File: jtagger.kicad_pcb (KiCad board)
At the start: 4 copper layers, 63 x 32 mm, 106 parts, among them J1 µUSB, J2 ARM_JTAG, J3 PADS, Q1 IRLML6402, Q2 IRLML6402, Q3 MMBT3906, Q4 2N7002, U1 MCP1700T-3302E/TT, U10 TPS61045DRB, U11 SI8642-QSOP, U2 SI8645-QSOP, U3 FT2232HQ, U4 EPM240-TQFP100, U5 MCP1700T-3302E/TT, U6 REE-0505S, U7 OSC-50MHz, U8 LTC1844ES5-3.3, U9 DG449DS, X1 12 MHz

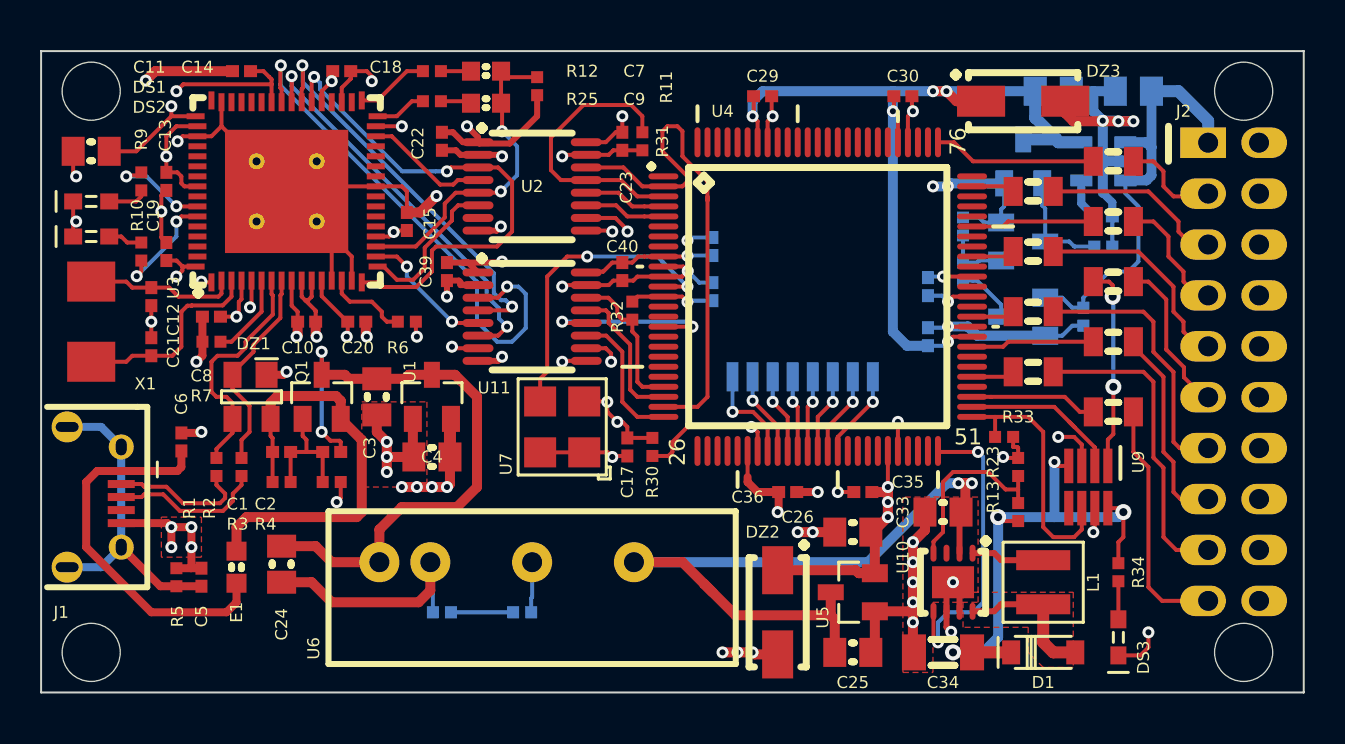
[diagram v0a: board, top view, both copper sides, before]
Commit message: Version submitted to fab
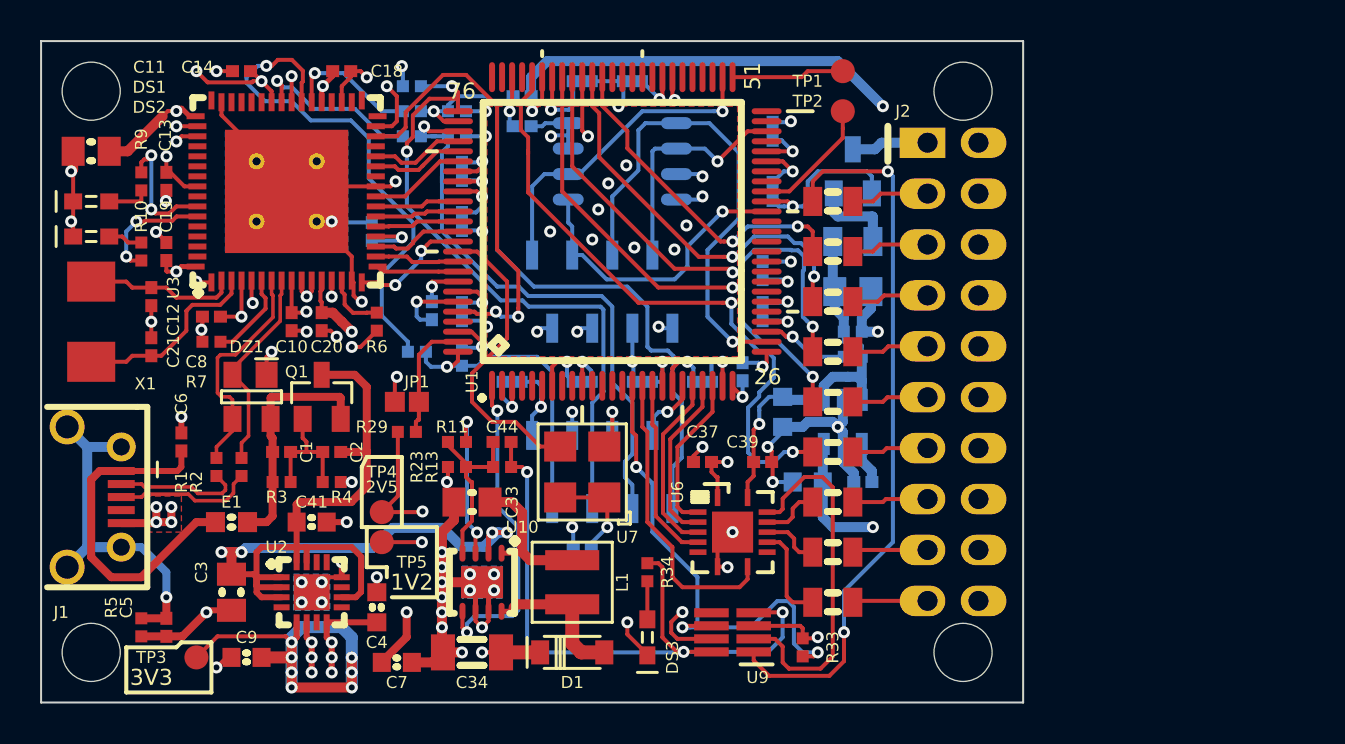
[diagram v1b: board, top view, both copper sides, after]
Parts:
- removed DZ2, DZ3: 1SMA5914BT3G, IPC7351-Nominal:DIOM5226X203
- removed Q3: MMBT3906, smd-semi:SOT-23
- removed Q4: 2N7002, smd-semi:SOT-23
- removed R32: 3k3, IPC7351-Nominal:RESC1005X40
- removed U11: SI8642-QSOP, IPC7351-Nominal:SOP63P600X160-16
- removed U8: LTC1844ES5-3.3, smd-semi:SOT-23-5
- added C41: 1u, IPC7351-Nominal:CAPC1608X55, F.Cu at (113.5, 111.5)
- added C42: 100n, IPC7351-Nominal:CAPC1005X55, B.Cu at (136.5, 95.0)
- added C43: 100n, IPC7351-Nominal:CAPC1005X55, B.Cu at (127.0, 89.5)
- added C44: 47p, IPC7351-Nominal:CAPC1005X55, F.Cu at (123.0, 107.5)
- added C45: 1u, IPC7351-Nominal:CAPC1608X55, B.Cu at (137.0, 106.0)
- added C46: 100n, IPC7351-Nominal:CAPC1005X55, B.Cu at (141.0, 109.5)
- added C47: 100n, IPC7351-Nominal:CAPC1005X55, B.Cu at (127.0, 112.8)
- added G***: LOGO, LOGO, B.Cu at (106.5, 109.0)
- added J4: JTAG, conn-molex:CONN-MOLEX-52808-0871, B.Cu at (128.0, 109.0)
- added JP1: PROGB, JUMPER-SOLDER, F.Cu at (118.2, 105.5)
- added R35: 10k, IPC7351-Nominal:RESC1005X40, B.Cu at (140.5, 102.0)
- added TP1: DONE, conn-test:TEST-SMD-SMALL, F.Cu at (140.0, 89.0)
- added TP2: INITB, conn-test:TEST-SMD-SMALL, F.Cu at (140.0, 91.0)
- added TP3: DONE, conn-test:TEST-SMD-SMALL, F.Cu at (107.8, 118.2)
- added TP4: DONE, conn-test:TEST-SMD-SMALL, F.Cu at (117.0, 111.0)
- added TP5: DONE, conn-test:TEST-SMD-SMALL, F.Cu at (117.0, 112.5)
- C12, C21: value 15p -> 3p3
- C15, C17, C22, C23, C29, C30, C35, C36, C40, R30: moved to B.Cu
- C24: value 10u -> 1u; footprint IPC7351-Nominal:CAPC2012X70 -> IPC7351-Nominal:CAPC1608X55; moved to B.Cu
- C25, C26: value 10u -> 100n; footprint IPC7351-Nominal:CAPC2012X70 -> IPC7351-Nominal:CAPC1005X55; moved to B.Cu
- C27: value 10u -> 100n; footprint IPC7351-Nominal:CAPC2012X70 -> IPC7351-Nominal:CAPC1005X55
- C37: moved to F.Cu
- C4: value 10u -> 1u; footprint IPC7351-Nominal:CAPC2012X70 -> IPC7351-Nominal:CAPC1608X55
- C7: value 100p -> 1u
- C9: value 1n -> 1u
- DS3: value LED-0603 -> LED
- DZ1: value SP0503BAHT -> DRTR5V0U2SR
- J3: value PADS -> FLASH
- R12: value 1k -> 10k; moved to B.Cu
- R13: value R-0402 -> 1M
- R23: value R-0402 -> 200k
- R24, R8: value 1M -> 0R
- R25: value 1k -> THERM; footprint IPC7351-Nominal:RESC1005X40 -> IPC7351-Nominal:RESC2012X50; moved to B.Cu
- R26, R27: value 3k3 -> 0R
- R28: value 3k3 -> 1k
- R29: value 3k3 -> 1k; moved to F.Cu
- R31: value 3k3 -> 1k; moved to B.Cu
- U1: value MCP1700T-3302E/TT -> XC3S50-VQ100; footprint smd-semi:SOT-23 -> IPC7351-Nominal:QFP50P1600X1600X100-100
- U2: value SI8645-QSOP -> ADP322ACPZ-145; footprint IPC7351-Nominal:SOP63P600X160-16 -> IPC7351-Nominal:QFN50P300X300X100-17
- U4: value EPM240-TQFP100 -> S25FL204; footprint IPC7351-Nominal:QFP50P1600X1600X160-100 -> IPC7351-Nominal:SOIC127P600X175-8; moved to B.Cu
- U5: value MCP1700T-3302E/TT -> LTC1844ES5-3.3; footprint smd-semi:SOT-23 -> smd-semi:SOT-23-5; moved to B.Cu
- U6: value REE-0505S -> TXB0104RGY; footprint manuf:RECOM-REE-0505S -> manuf:TEXAS-RGY
- moved R29 34.2 mm to (118.2, 107.0), turned to 0 degrees
- moved R28 32.9 mm to (120.8, 91.0)
- moved C27 32.9 mm to (119.5, 101.0), turned to 270 degrees
- moved C9 30.1 mm to (110.2, 118.2)
- moved C7 29.8 mm to (117.8, 118.5), turned to 0 degrees
- moved R26 28.4 mm to (118.5, 89.8), turned to 180 degrees
- moved R27 28.3 mm to (118.5, 92.2), turned to 180 degrees
- moved R23 28.0 mm to (120.8, 108.8), turned to 180 degrees
- moved C24 26.6 mm to (138.2, 109.5), turned to 180 degrees
- moved R13 25.8 mm to (123.0, 108.8), turned to 180 degrees
- moved R12 25.4 mm to (140.5, 103.2), turned to 0 degrees
- moved C26 25.0 mm to (129.5, 89.5)
- moved R8 25.0 mm to (118.5, 91.0), turned to 180 degrees
- moved C28 24.4 mm to (130.0, 104.5), turned to 180 degrees
- moved C31 24.0 mm to (121.0, 94.0)
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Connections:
- net /IN_OE renamed /AD11
- net Net-(U3-Pad26) renamed /AD8
- net Net-(U3-Pad34) renamed /AD15
- C16 pad 1: /VT_IN -> +VTGT
- C16 pad 2: (GND) -> GND
- C17 pad 1: (+3.3) -> /VTGTLIM
- C17 pad 2: (GND) -> GND
- C23 pad 1: (+3.3) -> +3.3
- C23 pad 2: (GND) -> GND
- C24 pad 1: +5 -> /VTGTLIM
- C25 pad 1: (+5) -> +2.5
- C25 pad 2: (GND) -> GND
- C26 pad 1: (+3.3) -> +2.5
- C26 pad 2: (GND) -> GND
- C27 pad 1: (+VTGT) -> +1.2
- C27 pad 2: (GND) -> GND
- C28 pad 1: Net-(C28-Pad1) -> +1.2
- C28 pad 2: (GND) -> GND
- C29 pad 1: (+VTGT) -> +3.3
- C29 pad 2: (GND) -> GND
- C30 pad 1: (+VTGT) -> +2.5
- C30 pad 2: (GND) -> GND
- C31 pad 1: (+3.3) -> +3.3
- C31 pad 2: (GND) -> GND
- C32 pad 1: (+VTGT) -> +2.5
- C32 pad 2: (GND) -> GND
- C33 pad 1: (+5) -> /SWL
- C33 pad 2: (GND) -> GND
- C34 pad 2: (GND) -> GND
- C35 pad 1: (+3.3) -> +3.3
- C35 pad 2: (GND) -> GND
- C36 pad 1: (+3.3) -> +3.3
- C36 pad 2: (GND) -> GND
- C37 pad 1: (+3.3) -> +3.3
- C37 pad 2: (GND) -> GND
- C38 pad 1: (+3.3) -> +3.3
- C38 pad 2: (GND) -> GND
- C39 pad 1: +3.3 -> +VTGT
- C4 pad 1: +3.3 -> +1.2
- C40 pad 1: (+3.3) -> +3.3
- C40 pad 2: (GND) -> GND
- C7 pad 1: /IN_TMS -> +2.5
- C7 pad 2: Net-(C7-Pad2) -> GND
- C9 pad 1: /IN_TMS -> +3.3
- C9 pad 2: Net-(C9-Pad2) -> GND
- DS3 pad 1: (GND) -> GND
- J2 pad 1: /VT_IN -> Net-(J2-Pad1)
- J2 pad 10: (GND) -> GND
- J2 pad 12: (GND) -> GND
- J2 pad 14: (GND) -> GND
- J2 pad 16: (GND) -> GND
- J2 pad 18: (GND) -> GND
- J2 pad 20: (GND) -> GND
- J2 pad 4: (GND) -> GND
- J2 pad 6: (GND) -> GND
- J2 pad 8: (GND) -> GND
- J3 pad 1: Net-(J3-Pad1) -> /CCLK
- J3 pad 2: Net-(J3-Pad2) -> +3.3
- J3 pad 3: Net-(J3-Pad3) -> /SPIMOSI
- J3 pad 4: Net-(J3-Pad4) -> GND
- J3 pad 5: Net-(J3-Pad5) -> /SPI#CS
- J3 pad 6: Net-(J3-Pad6) -> GND
- J3 pad 7: Net-(J3-Pad7) -> /SPIMISO
- J3 pad 8: Net-(J3-Pad8) -> GND
- Q2 pad 1: Net-(Q2-Pad1) -> GND
- Q2 pad 2: (+3.3) -> Net-(Q2-Pad2)
- Q2 pad 3: (+VTGT) -> Net-(J2-Pad1)
- R11 pad 1: +3.3 -> Net-(C44-Pad2)
- R11 pad 2: /IN_TMS -> Net-(R11-Pad2)
- R12 pad 1: Net-(C7-Pad2) -> /TGTSENSE
- R12 pad 2: Net-(R12-Pad2) -> +VTGT
- R13 pad 2: Net-(R13-Pad2) -> Net-(C44-Pad2)
- R14 pad 2: /TARG_#TRST -> Net-(R14-Pad2)
- R15 pad 2: /TARG_TDI -> /IN_TDI
- R16 pad 2: /TARG_TMS -> /IN_TMS
- R17 pad 2: /TARG_TCLKO -> /IN_TCK
- R18 pad 2: /AUX1_HVP -> /IN_RTCK
- R19 pad 2: /TARG_TDO -> /IN_TDO
- R20 pad 2: /TARG_#SRST -> Net-(R20-Pad2)
- R21 pad 2: /TARG_DBGREQ -> Net-(R21-Pad2)
- R22 pad 2: /TARG_DBGACK -> Net-(R22-Pad2)
- R23 pad 1: Net-(R13-Pad2) -> Net-(C44-Pad2)
- R23 pad 2: (GND) -> GND
- R24 pad 1: Net-(R24-Pad1) -> /FPGA_TDI
- R24 pad 2: (GND) -> Net-(R24-Pad2)
- R25 pad 1: Net-(C9-Pad2) -> Net-(Q2-Pad2)
- R25 pad 2: Net-(R25-Pad2) -> +VTGT
- R26 pad 1: (+3.3) -> /FPGA_TDO
- R26 pad 2: Net-(Q3-Pad1) -> Net-(R26-Pad2)
- R27 pad 1: Net-(Q3-Pad1) -> /FPGA_TMS
- R27 pad 2: Net-(Q4-Pad3) -> Net-(R27-Pad2)
- R28 pad 1: Net-(Q2-Pad1) -> /FPGA_TCK
- R28 pad 2: (GND) -> GND
- R29 pad 1: /VT_IN -> +2.5
- R29 pad 2: (GND) -> Net-(JP1-Pad1)
- R30 pad 1: /PC_TCK -> +3.3
- R30 pad 2: (GND) -> /FPGA_TMS
- R31 pad 1: /CPLD_SEL -> +3.3
- R31 pad 2: (GND) -> /FPGA_TDI
- R33 pad 1: Net-(R33-Pad1) -> /VPPEN
- R33 pad 2: (GND) -> GND
- R8 pad 1: GND -> /FPGA_TCK
- R8 pad 2: Net-(R24-Pad1) -> Net-(R8-Pad2)
- U1 pad 1: GND -> /VCTRL
- U1 pad 2: +3.3 -> Net-(U1-Pad2)
- U1 pad 3: +5 -> GND
- U10 pad 2: (+5) -> +5
- U10 pad 3: Net-(U10-Pad3) -> Net-(R11-Pad2)
- U10 pad 4: Net-(R13-Pad2) -> Net-(C44-Pad2)
- U10 pad 6: (GND) -> GND
- U10 pad 7: (GND) -> GND
- U10 pad 9: (GND) -> GND
- U2 pad 1: +3.3 -> +5
- U2 pad 10: (+3.3) -> +5
- U2 pad 11: /PC_TDI -> (no net)
- U2 pad 12: /PC_TMS -> GND
- U2 pad 13: /CPLD_SEL -> (no net)
- U2 pad 14: /PC_TCK -> (no net)
- U2 pad 15: (GND) -> +5
- U2 pad 16: (+3.3) -> +5
- U2 pad 2: GND -> +5
- U2 pad 3: /IN_TCK -> +5
- U2 pad 4: /IN_CPLD_SEL -> (no net)
- U2 pad 5: /IN_TMS -> +3.3
- U2 pad 6: /IN_TDI -> +2.5
- U2 pad 8: GND -> +1.2
- U2 pad 9: (GND) -> (no net)
- U3 pad 16: /IN_TCK -> /AD0
- U3 pad 17: /IN_TDI -> /AD1
- U3 pad 18: /IN_TDO -> /AD2
- U3 pad 19: /IN_TMS -> /AD3
- U3 pad 21: Net-(U3-Pad21) -> /AD4
- U3 pad 22: Net-(U3-Pad22) -> /AD5
- U3 pad 23: Net-(U3-Pad23) -> /AD6
- U3 pad 24: Net-(U3-Pad24) -> /AD7
- U3 pad 27: Net-(U3-Pad27) -> /AD9
- U3 pad 28: Net-(U3-Pad28) -> /AD10
- U3 pad 30: /IN_CPLD_SEL -> /AD12
- U3 pad 32: Net-(R25-Pad2) -> /AD13
- U3 pad 33: Net-(R12-Pad2) -> /AD14
- U3 pad 38: /IN_TCK -> Net-(R8-Pad2)
- U3 pad 39: /IN_CPLD_TDI -> Net-(R24-Pad2)
- U3 pad 40: /IN_CPLD_TDO -> Net-(R26-Pad2)
- U3 pad 41: /IN_CPLD_TMS -> Net-(R27-Pad2)
- U4 pad 1: Net-(U4-Pad1) -> /SPI#CS
- U4 pad 2: /PC_TCK -> /SPIMISO
- U4 pad 3: /CPLD_SEL -> +3.3
- U4 pad 4: /PC_TMS -> GND
- U4 pad 5: /PC_TDI -> /SPIMOSI
- U4 pad 6: Net-(U4-Pad6) -> /CCLK
- U4 pad 7: Net-(U4-Pad7) -> +3.3
- U4 pad 8: Net-(U4-Pad8) -> +3.3
- U5 pad 1: (GND) -> +VTGT
- U5 pad 2: (+3.3) -> GND
- U5 pad 3: (+5) -> +VTGT
- U6 pad 1: +5 -> +3.3
- U6 pad 2: GND -> /IN_#TRST
- U6 pad 4: (GND) -> /IN_DBGREQ
- U6 pad 6: (+5) -> (no net)
- U7 pad 1: (+3.3) -> +3.3
- U7 pad 2: (GND) -> GND
- U7 pad 3: /50MHz -> /50MHZ
- U7 pad 4: (+3.3) -> +3.3
- U9 pad 1: /AUX1_HVP -> Net-(R14-Pad2)
- U9 pad 2: Net-(U4-Pad52) -> Net-(U6-Pad13)
- U9 pad 3: (GND) -> GND
- U9 pad 6: Net-(R33-Pad1) -> /VPPEN
- U9 pad 7: (GND) -> GND
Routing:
- net GND: track 90.8 -> 243.4 mm, vias 27 -> 90
- net (GND): track 148.9 -> 0.00 mm, vias 35 -> 0
- net +1.2: track 0.00 -> 102.3 mm, vias 0 -> 8
- net +3.3: track 44.5 -> 142.1 mm, vias 14 -> 31
- net +2.5: track 0.00 -> 84.9 mm, vias 0 -> 9
- net /VTGTLIM: track 0.00 -> 50.4 mm, vias 0 -> 3
- net (+3.3): track 49.1 -> 0.00 mm, vias 13 -> 0
- net (+VTGT): track 44.8 -> 0.00 mm, vias 5 -> 0
- net (+5): track 37.4 -> 0.00 mm, vias 2 -> 0
- net Net-(R14-Pad2): track 0.00 -> 36.1 mm, vias 0 -> 2
- net /FPGA_TCK: track 0.00 -> 33.3 mm, vias 0 -> 1
- net /FPGA_TDO: track 0.00 -> 32.3 mm, vias 0 -> 2
- net /FPGA_TMS: track 0.00 -> 29.9 mm, vias 0 -> 1
- net /PC_TCK: track 29.8 -> 0.00 mm
- net /IN_CPLD_TMS: track 26.4 -> 0.00 mm, vias 2 -> 0
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- removed copper zone on Power, net (+3.3)
- removed copper zone on F.Cu, net (GND)
- removed copper zone on Ground, net (GND)
- removed copper zone on F.Cu, net /SW
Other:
- board size 63 x 32 mm -> 49 x 33 mm
- rule trace_min: 0.2 -> 0.16
- board text added: "1V2"
- board text added: "2V5"
- board text added: "3V3"
- board text removed: "33"
- board text removed: "40"
- board text removed: "DBGACK"
- board text removed: "DBGREQ"
- board text removed: "GND"
- board text removed: "ISOLATED PORT: UP TO 40V BETWEEN SIDES"
- board text removed: "RTCK"
- board text removed: "TCK"
- board text removed: "TDI"
- board text removed: "TDO"
- board text removed: "TMS"
- board text removed: "VTRG"
- board text removed: "~SRST"
- board text removed: "~TRST"
